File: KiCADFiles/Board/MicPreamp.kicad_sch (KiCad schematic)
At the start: 13 parts, among them U10 OPA1655D, U6 1512S08-U

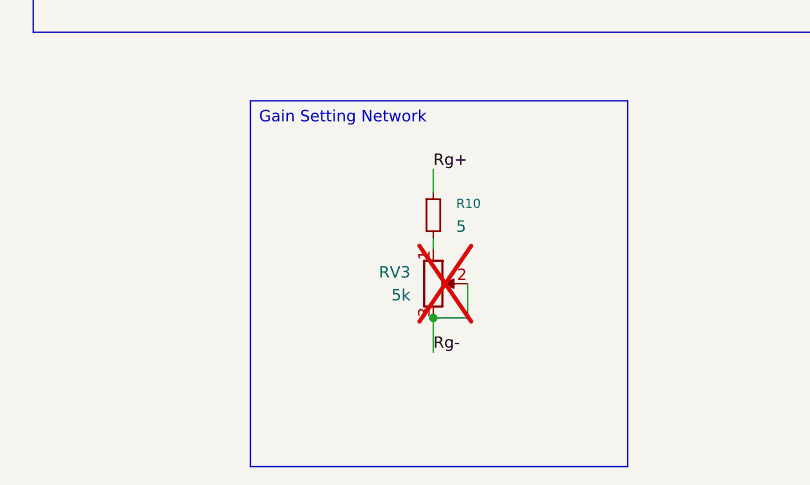
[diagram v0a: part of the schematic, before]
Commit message: improved layout further
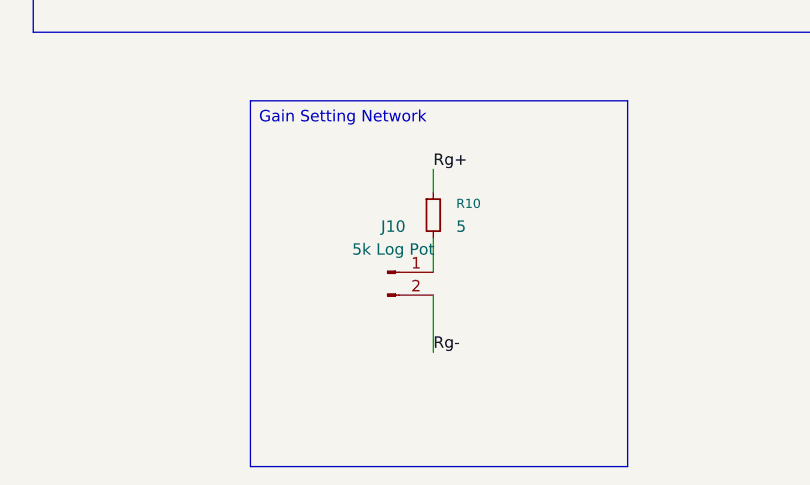
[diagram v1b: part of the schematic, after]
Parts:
- removed RV3: 5k, Potentiometer_THT:Potentiometer_Alps_RK163_Single_Horizontal, symbol Device:R_Potentiometer
- added J10: 5k Log Pot, Connector_PinHeader_2.54mm:PinHeader_1x02_P2.54mm_Vertical, symbol Connector:Conn_01x02_Pin
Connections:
- net Rg-: now also J10.2 (Pin_2)
- net at R10.2: now also J10.1 (Pin_1)
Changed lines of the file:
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@@
-	)
-	(junction
-		(at 160.02 121.92)
-		(diameter 0)
-		(color 0 0 0 0)
 	)
 	(junction
@@
 	(wire
 		(pts
-			(xy 163.83 121.92) (xy 160.02 121.92)
-		)
-		(stroke
-			(width 0)
-			(type default)
-		)
-	)
-	(wire
-		(pts
 			(xy 59.69 57.15) (xy 59.69 62.23)
 		)
@@
 	(wire
 		(pts
-			(xy 163.83 118.11) (xy 163.83 121.92)
-		)
-		(stroke
-			(width 0)
-			(type default)
-		)
-	)
-	(wire
-		(pts
 			(xy 156.21 74.93) (xy 177.8 74.93)
 		)
@@
 	(wire
 		(pts
-			(xy 160.02 121.92) (xy 160.02 125.73)
+			(xy 160.02 119.38) (xy 160.02 125.73)
 		)
 		(stroke
@@
 	(wire
 		(pts
-			(xy 160.02 113.03) (xy 160.02 114.3)
+			(xy 160.02 113.03) (xy 160.02 116.84)
 		)
 		(stroke
@@
 	)
 	(symbol
-		(lib_id "Device:R_Potentiometer")
-		(at 160.02 118.11 0)
-		(unit 1)
-		(exclude_from_sim no)
-		(in_bom yes)
-		(on_board yes)
-		(dnp yes)
-		(fields_autoplaced yes)
-		(property "Reference" "RV3"
-			(at 157.48 116.8399 0)
-			(effects
-				(font
-					(size 1.27 1.27)
-				)
-				(justify right)
-			)
-		)
-		(property "Value" "5k"
-			(at 157.48 119.3799 0)
-			(effects
-				(font
-					(size 1.27 1.27)
-				)
-				(justify right)
-			)
-		)
-		(property "Footprint" "Potentiometer_THT:Potentiometer_Alps_RK163_Single_Horizontal"
-			(at 160.02 118.11 0)
-			(effects
-				(font
-					(size 1.27 1.27)
-				)
-				(hide yes)
-			)
-		)
-		(property "Datasheet" "~"
-			(at 160.02 118.11 0)
-			(effects
-				(font
-					(size 1.27 1.27)
-				)
-				(hide yes)
-			)
-		)
-		(property "Description" "Potentiometer"
-			(at 160.02 118.11 0)
-			(effects
-				(font
-					(size 1.27 1.27)
-				)
-				(hide yes)
-			)
-		)
-		(property "MPN" "RV16AF-10-15K-C5K-3LA "
-			(at 160.02 118.11 0)
-			(effects
-				(font
-					(size 1.27 1.27)
-				)
-				(hide yes)
-			)
-		)
-		(property "Tol" ""
-			(at 160.02 118.11 0)
-			(effects
-				(font
-					(size 1.27 1.27)
-				)
-				(hide yes)
-			)
-		)
-		(pin "3"
-		)
-		(pin "2"
-		)
-		(pin "1"
-		)
-		(instances
-			(project "SuperAudioBoard"
-				(path "/01f65e03-4e05-4001-87b4-b3e88e4198ab/00000000-0000-0000-0000-00005438c479/cc56b259-b7b6-4889-861e-4cceeb5868cc"
-					(reference "RV3")
-					(unit 1)
-				)
-			)
-		)
-	)
-	(symbol
 		(lib_id "Amplifier_Operational:OPA1655D")
 		(at 62.23 69.85 0)
@@
 					(unit 1)
 				)
+			)
+		)
+	)
+	(symbol
+		(lib_id "Connector:Conn_01x02_Pin")
+		(at 154.94 116.84 0)
+		(unit 1)
+		(exclude_from_sim no)
+		(in_bom yes)
+		(on_board yes)
+		(dnp no)
+		(fields_autoplaced yes)
+		(property "Reference" "J10"
+			(at 155.575 111.76 0)
+			(effects
+				(font
+					(size 1.27 1.27)
+				)
+			)
+		)
+		(property "Value" "5k Log Pot"
+			(at 155.575 114.3 0)
+			(effects
+				(font
+					(size 1.27 1.27)
+				)
+			)
+		)
+		(property "Footprint" "Connector_PinHeader_2.54mm:PinHeader_1x02_P2.54mm_Vertical"
+			(at 154.94 116.84 0)
+			(effects
+				(font
+					(size 1.27 1.27)
+				)
+				(hide yes)
+			)
+		)
+		(property "Datasheet" "~"
+			(at 154.94 116.84 0)
+			(effects
+				(font
+					(size 1.27 1.27)
+				)
+				(hide yes)
+			)
+		)
+		(property "Description" "Generic connector, single row, 01x02, script generated"
+			(at 154.94 116.84 0)
+			(effects
+				(font
+					(size 1.27 1.27)
+				)
+				(hide yes)
+			)
+		)
+		(property "MPN" "RV16AF-10-15K-C5K-3LA "
+			(at 154.94 116.84 0)
+			(effects
+				(font
+					(size 1.27 1.27)
+				)
+				(hide yes)
+			)
+		)
+		(pin "2"
+		)
+		(pin "1"
+		)
+		(instances
+			(project "SuperAudioBoard"
+				(path "/01f65e03-4e05-4001-87b4-b3e88e4198ab/00000000-0000-0000-0000-00005438c479/cc56b259-b7b6-4889-861e-4cceeb5868cc"
+					(reference "J10")
+					(unit 1)
+				)
